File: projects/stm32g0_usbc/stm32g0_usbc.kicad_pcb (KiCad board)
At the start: 2 copper layers, 33.3 x 24.6 mm, 26 parts, among them J1 USB_C_Receptacle_USB2.0, J3 Conn_ARM_JTAG_SWD_10, U1 STM32G0B1CBT, U2 MCP1754S-3302xMB, Y2 NX3225GD 8 MHz

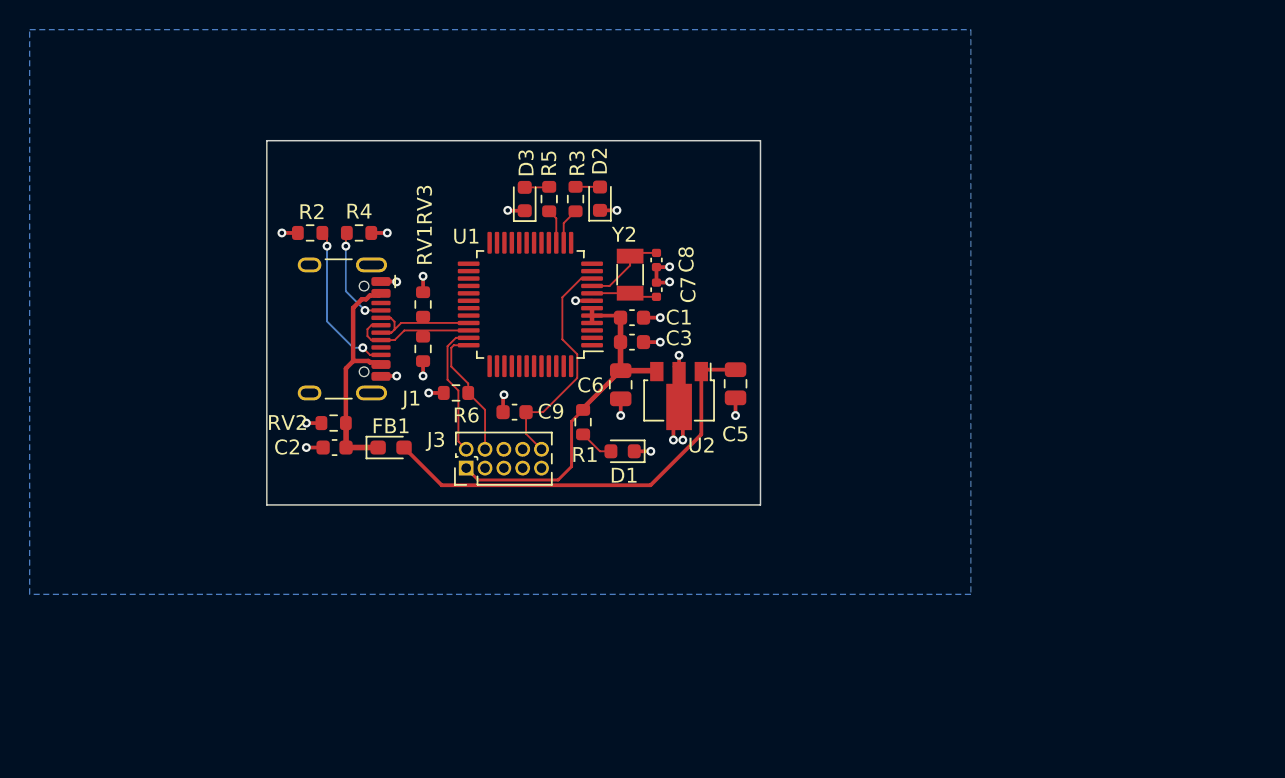
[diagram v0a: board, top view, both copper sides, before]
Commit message: .
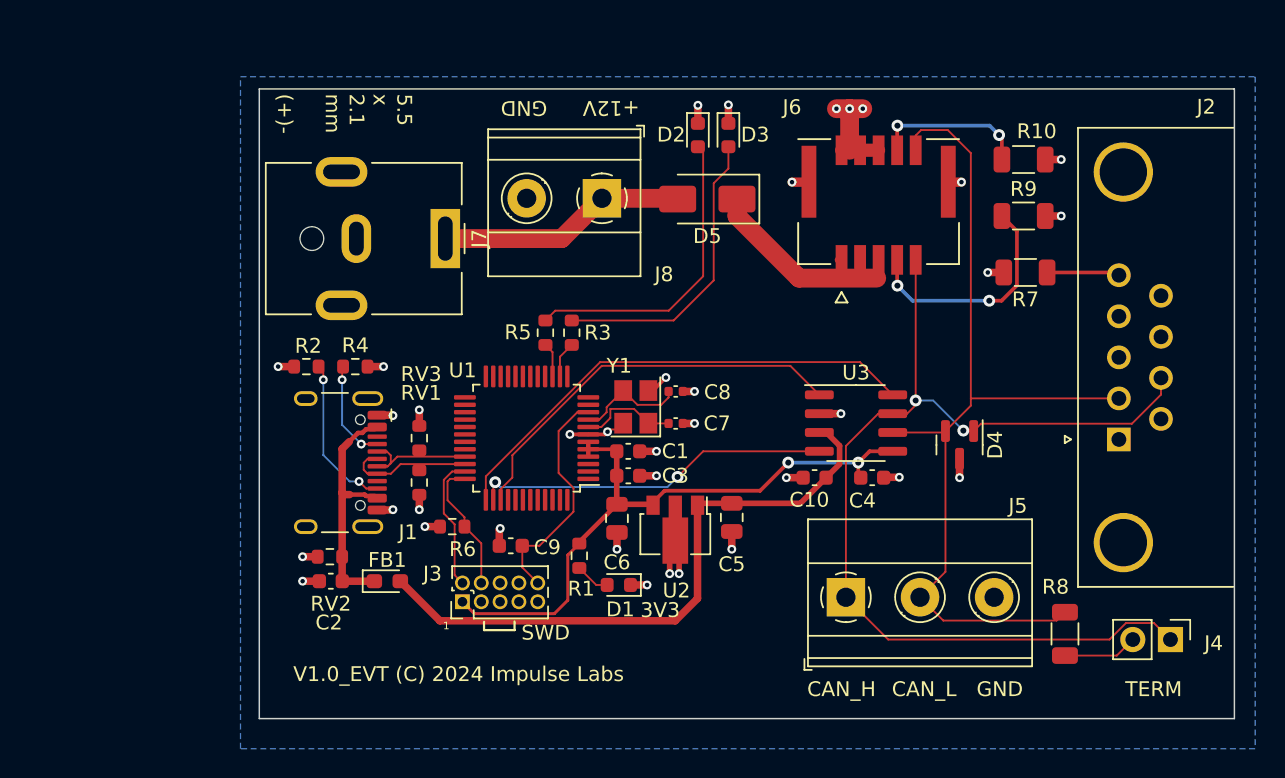
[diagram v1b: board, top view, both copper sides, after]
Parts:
- removed Y2: NX3225GD 8 MHz, Crystal:Crystal_SMD_3215-2Pin_3.2x1.5mm
- added C10: 100n, Capacitor_SMD:C_0603_1608Metric, F.Cu at (116.5, 81.0)
- added C4: 100n, Capacitor_SMD:C_0603_1608Metric, F.Cu at (120.3, 81.0)
- added D4: NUP2105L, Package_TO_SOT_SMD:SOT-23, F.Cu at (126.2, 78.8)
- added D5: D_Schottky, Diode_SMD:D_SMA, F.Cu at (109.2, 62.2)
- added J2: DE9_Plug, Connector_Dsub:DSUB-9_Male_Horizontal_P2.77x2.84mm_EdgePinOffset4.94mm_Housed_MountingHolesOffset7.48mm, F.Cu at (137.0, 78.4)
- added J4: Conn_01x02, Connector_PinHeader_2.54mm:PinHeader_1x02_P2.54mm_Vertical, F.Cu at (140.5, 91.9)
- added J5: Screw_Terminal_01x03, TerminalBlock_Phoenix:TerminalBlock_Phoenix_MKDS-1,5-3_1x03_P5.00mm_Horizontal, F.Cu at (118.6, 89.1)
- added J6: 5054481071, molex_microlock_plus:MOLEX_5054481071, F.Cu at (120.8, 62.6)
- added J7: Conn_Coaxial_Power, Connector_BarrelJack:BarrelJack_CUI_PJ-063AH_Horizontal, F.Cu at (91.5, 64.9)
- added J8: Screw_Terminal_01x02, TerminalBlock_Phoenix:TerminalBlock_Phoenix_MKDS-1,5-2-5.08_1x02_P5.08mm_Horizontal, F.Cu at (102.1, 62.2)
- added R10: 0, Resistor_SMD:R_1206_3216Metric, F.Cu at (130.6, 59.6)
- added R7: DNI, Resistor_SMD:R_1206_3216Metric, F.Cu at (130.7, 67.2)
- added R8: 120, Resistor_SMD:R_1206_3216Metric, F.Cu at (133.3, 91.6)
- added R9: 0, Resistor_SMD:R_1206_3216Metric, F.Cu at (130.6, 63.4)
- added U3: TJA1051T-3, Package_SO:SOIC-8_3.9x4.9mm_P1.27mm, F.Cu at (119.3, 77.3)
- added Y1: Crystal_GND24_Small, Crystal:Crystal_SMD_3225-4Pin_3.2x2.5mm, F.Cu at (104.4, 76.3)
- moved D3 12.5 mm to (108.6, 57.9), turned to -90 degrees
- moved D2 9.67 mm to (110.6, 57.9), turned to -90 degrees
- moved C7 9.11 mm to (107.1, 77.4), turned to 0 degrees
- moved C1 9.02 mm to (103.9, 79.2)
- moved C9 9.02 mm to (96.0, 85.6)
- moved J1 9.02 mm to (83.2, 80.0)
- moved R3 9.02 mm to (100.1, 71.2)
- moved R5 9.02 mm to (98.3, 71.2)
- moved C2 9.02 mm to (83.8, 88.0)
- moved C3 9.02 mm to (103.9, 80.9)
- moved C5 9.02 mm to (110.9, 83.7)
- moved C6 9.02 mm to (103.1, 83.8)
- moved D1 9.02 mm to (103.3, 88.3)
- moved FB1 9.02 mm to (87.6, 88.0)
- moved J3 9.02 mm to (92.7, 89.4)
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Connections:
- U1 pad 37: unconnected-(U1A-PA15-Pad37) -> /CAN1_S
- U1 pad 38: unconnected-(U1D-PD0-Pad38) -> /CAN1_RX
- U1 pad 39: unconnected-(U1D-PD1-Pad39) -> /CAN1_TX
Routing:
- net /CAN1_H: track 0.00 -> 69.4 mm, vias 0 -> 2
- net /CAN1_L: track 0.00 -> 61.2 mm
- net /CAN1_S: track 0.00 -> 33.1 mm
- net /CAN1_TX: track 0.00 -> 27.4 mm
- net /CAN1_RX: track 0.00 -> 24.2 mm, vias 0 -> 2
- net Net-(D3-A): track 1.67 -> 20.8 mm
- net +3V3: track 24.0 -> 42.8 mm, vias 0 -> 2
- net Net-(D2-A): track 1.66 -> 20.1 mm
- net GND: track 26.6 -> 44.5 mm, vias 23 -> 36
- net /+12V_IN: track 0.00 -> 16.8 mm
- net /12V_SHIELD: track 0.00 -> 15.8 mm, vias 0 -> 2
- net +12V: track 0.00 -> 12.5 mm
- net +5V: track 29.1 -> 41.1 mm
- net /SHIELD: track 0.00 -> 10.5 mm, vias 0 -> 2
- net Net-(J4-Pin_2): track 0.00 -> 5.02 mm
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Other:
- board size 33.3 x 24.6 mm -> 65.8 x 42.5 mm
- board text added: "+12V"
- board text added: "1"
- board text added: "3V3"
- board text added: "5.5 x 2.1 mm (+)-"
- board text added: "CAN_H"
- board text added: "CAN_L"
- board text added: "GND"
- board text added: "SWD"
- board text added: "TERM"
- board text added: "V1.0_EVT (C) 2024 Impulse Labs"
